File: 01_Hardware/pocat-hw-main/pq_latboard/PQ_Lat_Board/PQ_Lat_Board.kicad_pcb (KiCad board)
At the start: 6 copper layers, 48 x 48 mm, 27 parts, among them IC1 TCN75AVOA713, J1 Conn_01x11_MountingPin, J2 Conn_Coaxial

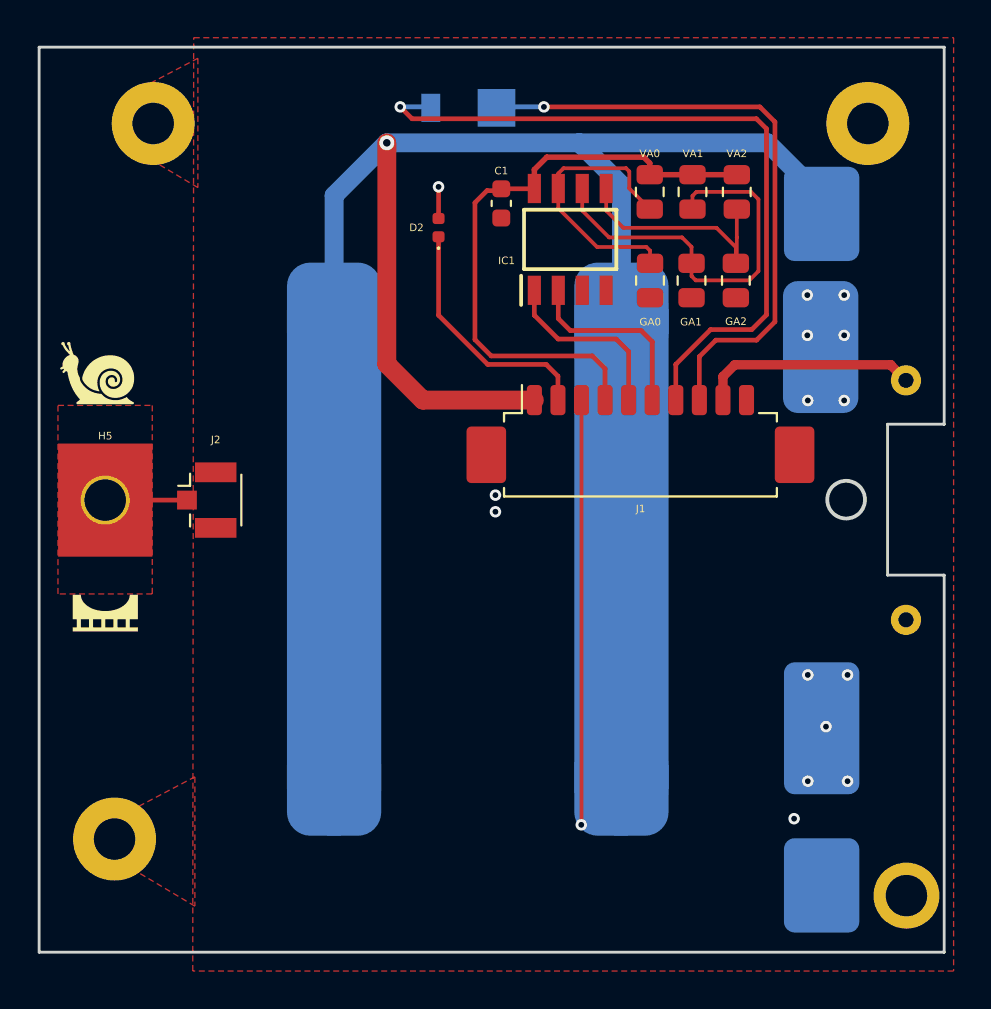
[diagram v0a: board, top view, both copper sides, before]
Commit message: Pcbs actualizados corregidos (son definitivos para mandarlos a fabricar con sus respectivos Gebers en una carpeta separada)
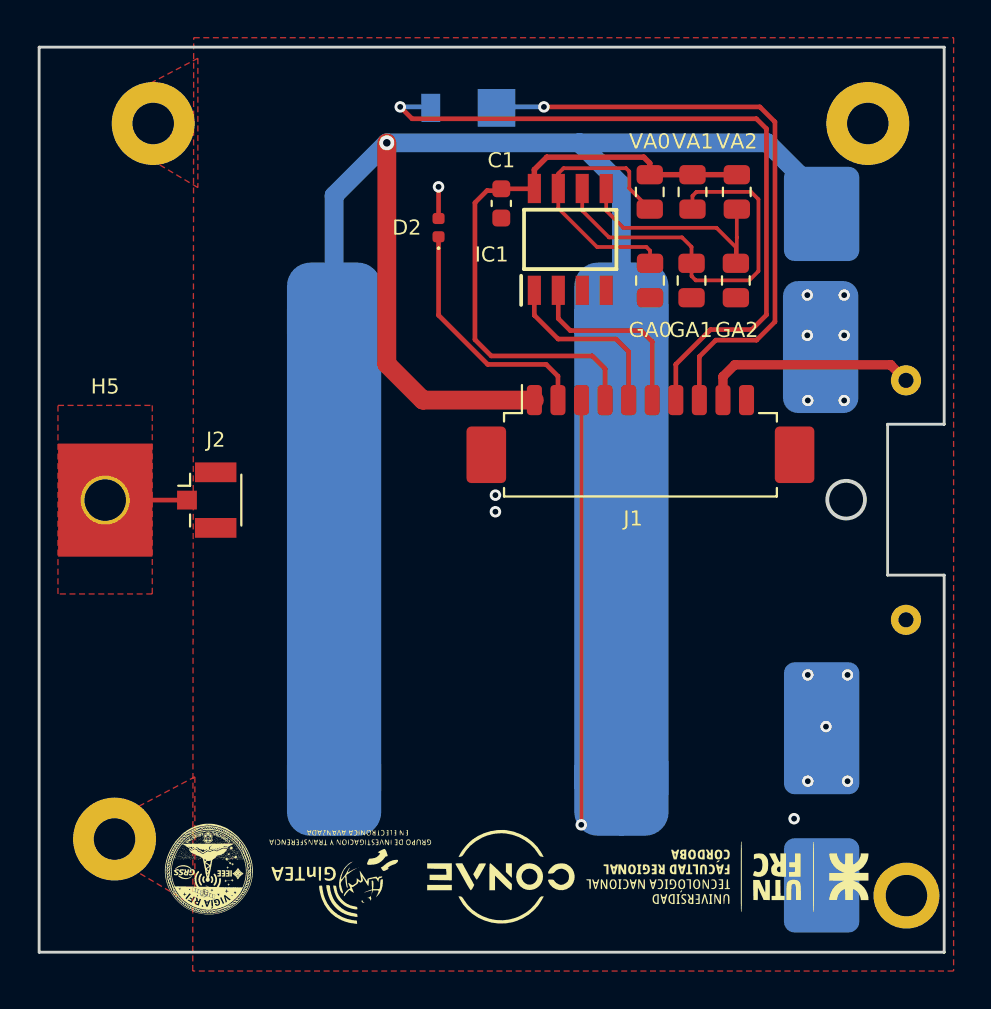
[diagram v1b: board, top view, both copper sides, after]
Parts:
- removed Annotation1: bridgemaker, symbols-nsl:Bridgemaker
- removed Annotation2: snail, symbols-nsl:Snail
- removed Annotation5: telecos, symbols-nsl:Telecos
- removed Annotation7: UPC, symbols-nsl:UPC_small
- removed Annotation8: GRSS, symbols-nsl:GRSS
- added G***: LOGO, LOGO, F.Cu at (91.5, 86.0)
- added G***: LOGO, LOGO, F.Cu at (111.5, 86.0)
- added G***: LOGO, LOGO, F.Cu at (99.5, 86.0)
- added G***: LOGO, LOGO, F.Cu at (84.0, 85.5)
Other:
- board text removed: "Adriano Camps Ştefan Podaru Guillem Gràcia Solá Marc Corretgé Artur Cot Arnau Dolz Edgar Hernández Roger Almirall Júlia Alós Óscar Pavón Nil Rius Júlia Tribó"
